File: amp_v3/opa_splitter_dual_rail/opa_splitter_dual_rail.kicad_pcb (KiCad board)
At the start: 2 copper layers, 62.9 x 30.5 mm, 19 parts, among them J6 PWR_IN, J7 AUDIO_IN, J8 AOUT_MASTER, J9 AOUT_VIS, U2 OPA1656

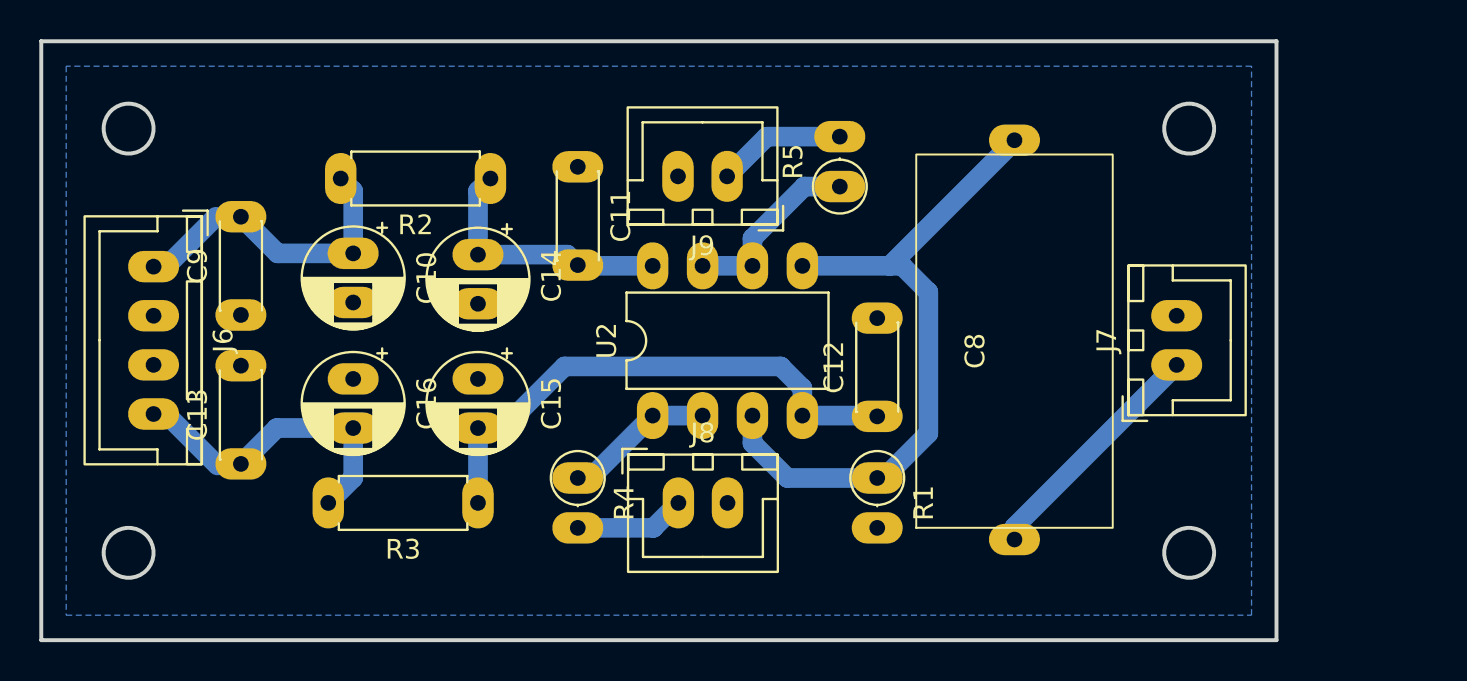
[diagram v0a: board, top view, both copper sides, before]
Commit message: updates
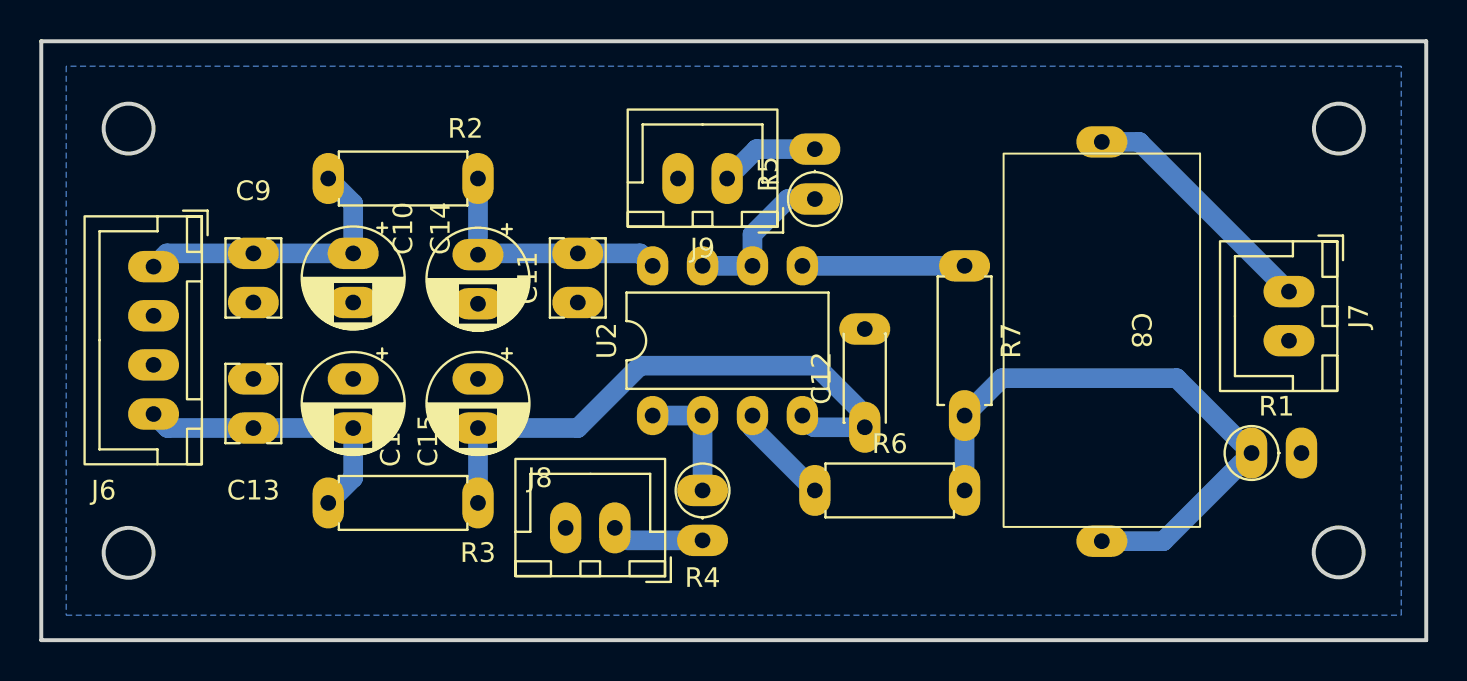
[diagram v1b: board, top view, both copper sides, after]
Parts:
- added R6: 100R, Resistor_THT:R_Axial_DIN0207_L6.3mm_D2.5mm_P7.62mm_Horizontal, F.Cu at (64.1, 95.2)
- added R7: 100R, Resistor_THT:R_Axial_DIN0207_L6.3mm_D2.5mm_P7.62mm_Horizontal, F.Cu at (71.8, 83.8)
- C11, C13, C9: footprint Capacitor_THT:C_Disc_D4.3mm_W1.9mm_P5.00mm -> Capacitor_THT:C_Disc_D3.8mm_W2.6mm_P2.50mm
- J7: value AUDIO_IN -> RCA_IN
- J8: value AOUT_MASTER -> AOUT_VACTROL
- moved C8 24.5 mm to (78.7, 75.6), turned to -90 degrees
- moved R1 19.1 mm to (86.4, 93.3), turned to 0 degrees
- moved C11 6.91 mm to (52.1, 85.7), turned to 90 degrees
- moved J7 6.82 mm to (88.3, 85.1), turned to -90 degrees
- moved R4 6.38 mm to (58.4, 95.2)
- moved J8 3.48 mm to (54.0, 97.2), turned to 180 degrees
- moved C13 1.93 mm to (35.6, 92.1)
- moved R5 1.42 mm to (64.1, 80.4)
- moved C9 0.90 mm to (35.6, 85.7)
- moved C12 0.84 mm to (66.7, 92.0)
- moved R2 0.63 mm to (47.0, 79.4)
- moved J9 0.11 mm to (59.7, 79.4)
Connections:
- U2 pad 3: /AUDIO_IN -> Net-(U2A-+)
- U2 pad 5: /AUDIO_IN -> Net-(U2B-+)
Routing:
- net Net-(U2B-+): track 0.00 -> 8.25 mm
- net /AUDIO_IN: track 36.1 -> 30.9 mm
- net Net-(U2A-+): track 0.00 -> 5.13 mm
- net Net-(U2C-V-): track 26.8 -> 30.0 mm
- net /AUDIO_OUT_MASTER: track 6.57 -> 5.08 mm
- net Net-(U2B--): track 9.48 -> 8.06 mm
- net Net-(U2A--): track 7.82 -> 6.51 mm
- net /RCA_IN: track 12.3 -> 13.3 mm
- net /AUDIO_OUT_VACTROL: track 5.65 -> 4.73 mm
- net /-12VA: track 14.5 -> 13.6 mm
- net /+12VA: track 14.2 -> 14.8 mm
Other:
- board size 62.9 x 30.5 mm -> 70.5 x 30.5 mm
